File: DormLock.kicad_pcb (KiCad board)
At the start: 2 copper layers, 84.9 x 81.7 mm, 68 parts, among them J1 Conn_02x03_Odd_Even, J10 Conn_02x03_Odd_Even, J2 Conn_01x05, J4 Conn_01x03, J5 Conn_01x02, J6 Conn_01x15, J7 Conn_01x15, J8 Conn_01x08, J9 USB_C_Receptacle, Q1 Q_NPN_BEC, Q2 Q_PMOS_GSD, Q3 Q_PMOS_GSD, SW1 SW_Push, U1 SPX1117M3-L-3-3/TR, U2 SY8105, U3 STM32F030CCTx, U4 LM321

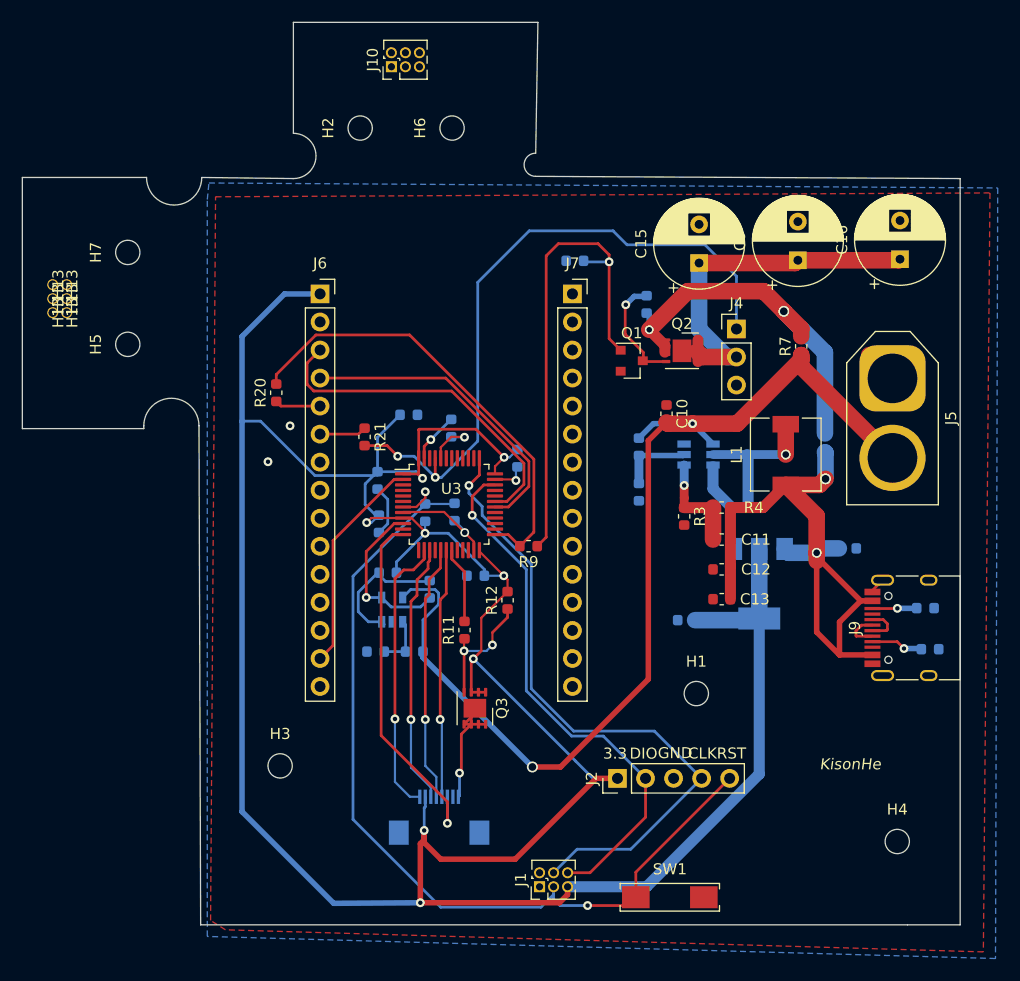
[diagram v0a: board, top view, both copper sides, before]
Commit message: PCBV3.0
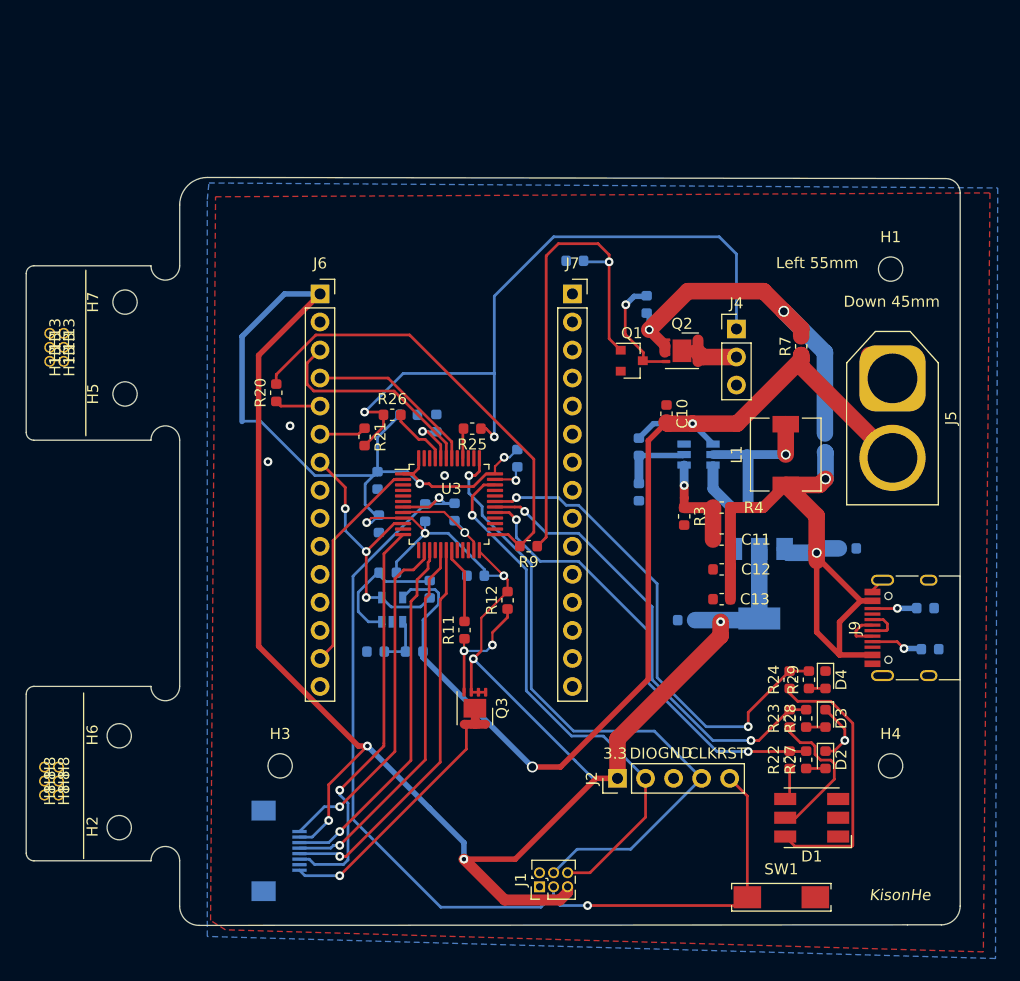
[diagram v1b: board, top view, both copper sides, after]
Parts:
- removed C15, C9: 470uf, Capacitor_THT:CP_Radial_D8.0mm_P3.50mm
- removed C16: 1000uf, Capacitor_THT:CP_Radial_D8.0mm_P3.50mm
- removed the H13 at (117.8, 81.7)
- removed the H13 at (117.8, 83.0)
- removed the H13 at (117.8, 84.2)
- removed the H13 at (116.5, 81.7)
- removed the H13 at (116.5, 83.0)
- removed the H13 at (116.5, 84.2)
- removed J10: Conn_02x03_Odd_Even, Connector_PinHeader_1.27mm:PinHeader_2x03_P1.27mm_Vertical
- added D1: LED_RGB, LED_SMD:LED_RGB_5050-6, F.Cu at (185.2, 130.0)
- added D2: LED, LED_SMD:LED_0603_1608Metric, F.Cu at (186.5, 124.8)
- added D3: LED, LED_SMD:LED_0603_1608Metric, F.Cu at (186.5, 121.0)
- added D4: LED, LED_SMD:LED_0603_1608Metric, F.Cu at (186.5, 117.5)
- added H13: 0.7mm Hole, KisonCommon:0.7mmInR Hole, F.Cu at (116.2, 88.7)
- added H13: 0.7mm Hole, KisonCommon:0.7mmInR Hole, F.Cu at (117.5, 88.7)
- added H13: 0.7mm Hole, KisonCommon:0.7mmInR Hole, F.Cu at (116.2, 87.4)
- added H13: 0.7mm Hole, KisonCommon:0.7mmInR Hole, F.Cu at (117.5, 87.4)
- added H13: 0.7mm Hole, KisonCommon:0.7mmInR Hole, F.Cu at (116.2, 86.1)
- added H13: 0.7mm Hole, KisonCommon:0.7mmInR Hole, F.Cu at (117.5, 86.1)
- added H8: 0.7mm Hole, KisonCommon:0.7mmInR Hole, F.Cu at (115.8, 127.9)
- added H8: 0.7mm Hole, KisonCommon:0.7mmInR Hole, F.Cu at (117.0, 127.9)
- added H8: 0.7mm Hole, KisonCommon:0.7mmInR Hole, F.Cu at (115.8, 126.7)
- added H8: 0.7mm Hole, KisonCommon:0.7mmInR Hole, F.Cu at (117.0, 126.7)
- added H8: 0.7mm Hole, KisonCommon:0.7mmInR Hole, F.Cu at (115.8, 125.4)
- added H8: 0.7mm Hole, KisonCommon:0.7mmInR Hole, F.Cu at (117.0, 125.4)
- added R22: 2.2k, Resistor_SMD:R_0603_1608Metric, F.Cu at (183.2, 124.8)
- added R23: 2.2k, Resistor_SMD:R_0603_1608Metric, F.Cu at (183.2, 121.0)
- added R24: 2.2k, Resistor_SMD:R_0603_1608Metric, F.Cu at (183.2, 117.5)
- added R25: 0, Resistor_SMD:R_0603_1608Metric, F.Cu at (154.5, 94.8)
- added R26: 0, Resistor_SMD:R_0603_1608Metric, F.Cu at (147.2, 93.5)
- added R27: 2.2k, Resistor_SMD:R_0603_1608Metric, F.Cu at (184.8, 124.8)
- added R28: 2.2k, Resistor_SMD:R_0603_1608Metric, F.Cu at (184.8, 121.0)
- added R29: 2.2k, Resistor_SMD:R_0603_1608Metric, F.Cu at (185.0, 117.5)
- R20, R21: footprint Capacitor_SMD:C_0603_1608Metric -> Resistor_SMD:R_0603_1608Metric
- moved H2 67.0 mm to (122.5, 130.9), turned to 180 degrees
- moved H6 62.8 mm to (122.5, 122.6), turned to 180 degrees
- moved H1 42.3 mm to (192.4, 80.3)
- moved J8 14.8 mm to (137.0, 133.0), turned to 90 degrees
- moved SW1 10.1 mm to (182.5, 137.2)
- moved H4 6.88 mm to (192.4, 125.3)
- moved H7 4.51 mm to (123.0, 83.3)
- moved H5 4.50 mm to (123.0, 91.6)
- moved R8 1.42 mm to (151.2, 94.2)
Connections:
- J6 pad 7: Net-(J6-Pad7) -> /BATT_AD
- U3 pad 29: Net-(U3-Pad29) -> /RGB_B
- U3 pad 30: /UART_32TX -> /RGB_G
- U3 pad 31: /UART_32RX -> /RGB_R
- U3 pad 42: Net-(U3-Pad42) -> /UART_32TX
- U3 pad 43: Net-(U3-Pad43) -> /UART_32RX
- U3 pad 45: /STEER_PWM -> Net-(R26-Pad2)
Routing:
- net /RGB_R: track 0.00 -> 45.2 mm, vias 0 -> 2
- net /RGB_G: track 0.00 -> 42.0 mm, vias 0 -> 2
- net /RGB_B: track 0.00 -> 40.9 mm, vias 0 -> 2
- net /VOutput: track 39.7 -> 10.9 mm
- net Net-(D1-Pad6): track 0.00 -> 24.9 mm
- net +3V3: track 270.7 -> 250.1 mm, vias 8 -> 10
- net /LEDA: track 12.4 -> 26.7 mm
- net Net-(D1-Pad5): track 0.00 -> 13.4 mm
- net /DC: track 22.6 -> 35.8 mm
- net /UART_32TX: track 28.2 -> 15.8 mm
- net /UART_32RX: track 31.4 -> 19.8 mm
- net /SDA: track 23.3 -> 34.3 mm
- net /STM_NRST: track 83.3 -> 93.3 mm
- net /BATT_AD: track 15.0 -> 24.8 mm, vias 1 -> 3
- net /SCL: track 23.8 -> 32.9 mm
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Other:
- board size 84.9 x 81.7 mm -> 84.6 x 67.8 mm
- board text added: "Down 45mm"
- board text added: "Left 55mm"
